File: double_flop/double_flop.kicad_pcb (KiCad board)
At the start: 2 copper layers, 55.8 x 70 mm, 8 parts, among them J1 Conn_01x04, SW1 Button 1, SW2 Button 2, SW3 Button 3, SW4 Button 4, U1 STM32F401, U2 CR2013-MI2120

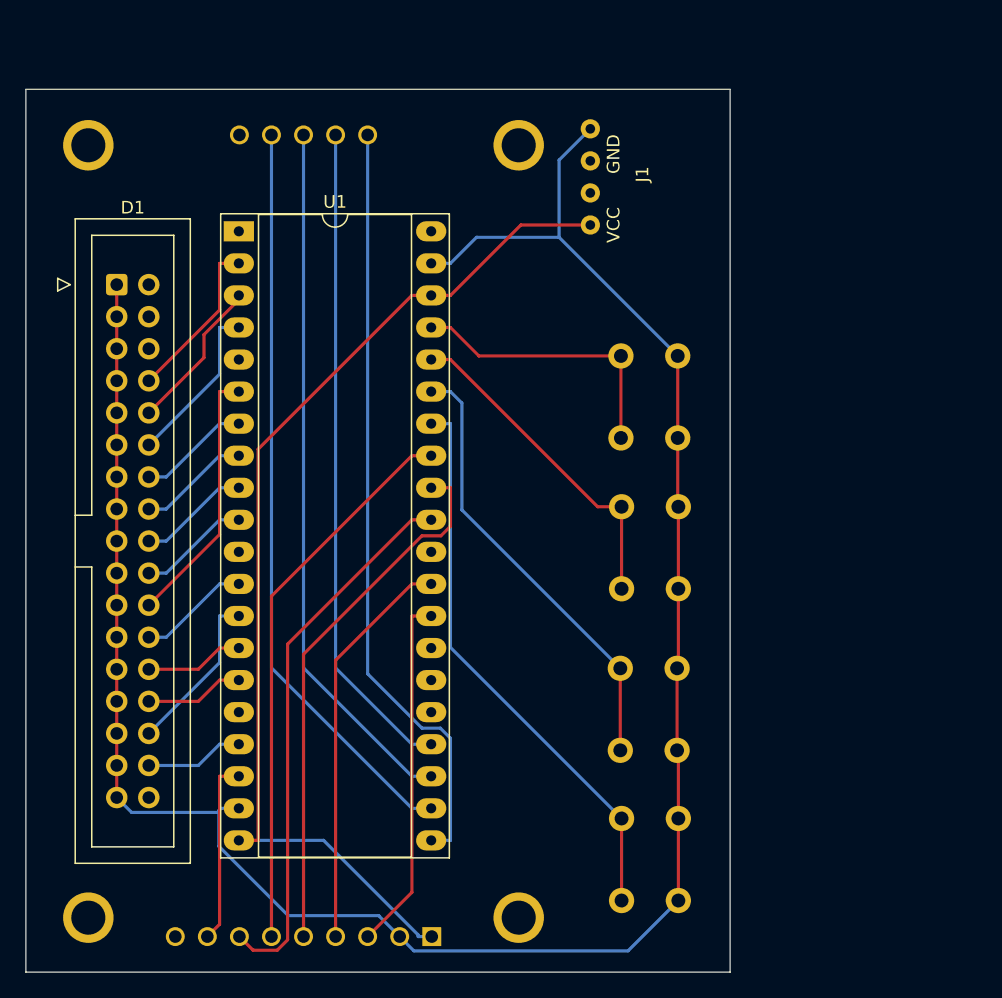
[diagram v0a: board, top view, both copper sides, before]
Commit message: Update 08042024
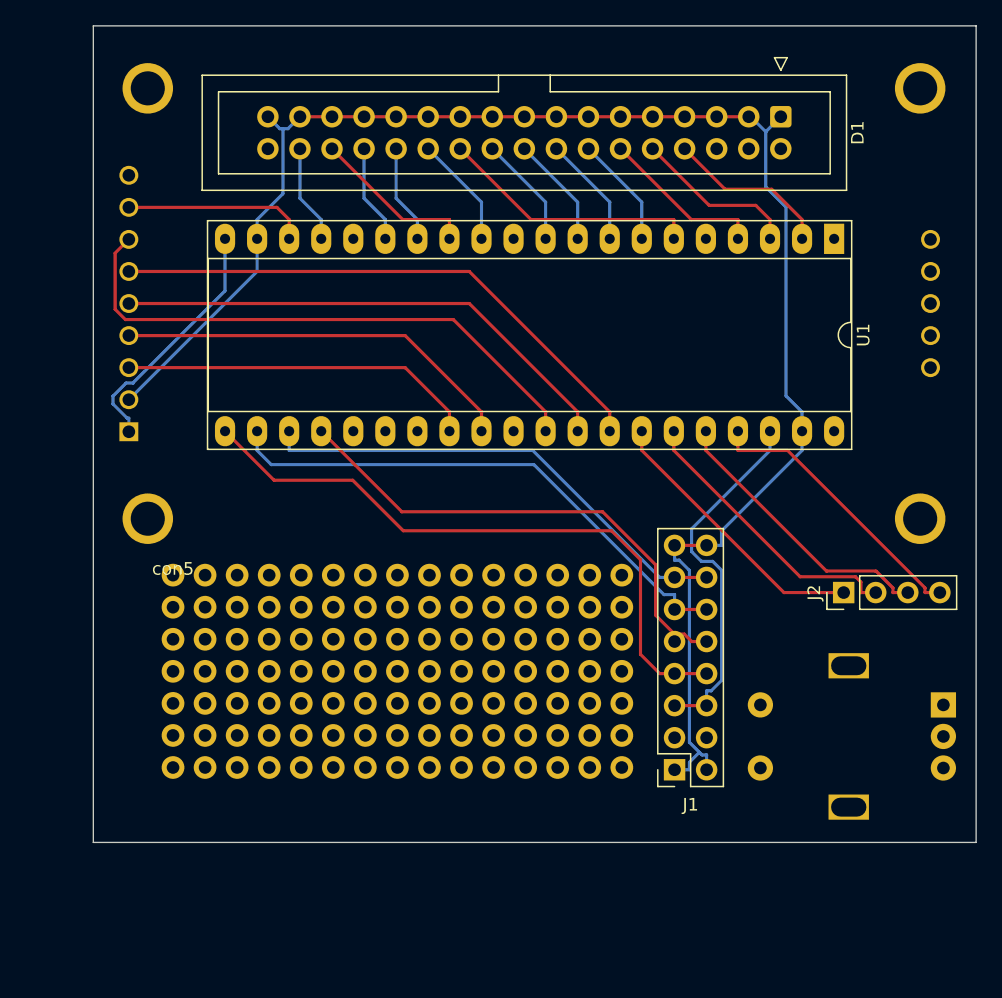
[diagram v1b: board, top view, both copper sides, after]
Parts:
- removed SW1: Button 1, Button_Switch_THT:SW_PUSH_6mm
- removed SW2: Button 2, Button_Switch_THT:SW_PUSH_6mm
- removed SW3: Button 3, Button_Switch_THT:SW_PUSH_6mm
- removed SW4: Button 4, Button_Switch_THT:SW_PUSH_6mm
- added J2: Conn_01x04_Pin, Double_flop_lib:PinHeader_1x04_P2.54mm_Vertical, F.Cu at (193.9, 67.5)
- added con5: Devboard, Double_flop:Devboard, F.Cu at (140.8, 66.1)
- added con6: RotaryEncoder_Alps_EC11E-Switch_Vertical_H20mm, Double_flop_lib:RotaryEncoder_Alps_EC11E-Switch_Vertical_H20mm, B.Cu at (201.8, 76.4)
- D1: footprint Connector_IDC:IDC-Header_2x17_P2.54mm_Vertical -> Double_flop_lib:IDC-Header_2x17_P2.54mm_Vertical
- J1: value Conn_01x04 -> SDCard Adapter; footprint Double_flop:USB-C Power board -> Double_flop_lib:PinSocket_2x08_P2.54mm_Vertical
- U1: footprint Package_DIP:DIP-40_W15.24mm_Socket_LongPads -> Double_flop_lib:DIP-40_W15.24mm_Socket_LongPads
- U2: footprint Display:CR2013-MI2120 -> Double_flop_lib:CR2013-MI2120
- moved D1 54.3 mm to (188.9, 29.8), turned to -90 degrees
- moved J1 47.5 mm to (180.5, 81.5), turned to 180 degrees
- moved U1 47.2 mm to (193.1, 39.5), turned to -90 degrees
- moved U2 46.6 mm to (137.3, 54.8), turned to 0 degrees
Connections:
- J1 pad 1: +5V -> GND
- J1 pad 2: unconnected-(J1-Pin_2-Pad2) -> GND
- J1 pad 4: GND -> unconnected-(J1-Pin_4-Pad4)
- U1 pad 20: +5V -> Net-(U2-VCC)
- U2 pad 1: +5V -> Net-(U2-VCC)
- U2 pad 10: SS -> unconnected-(U2-SD_CS-Pad10)
- U2 pad 11: MOSI -> unconnected-(U2-SD_MOSI-Pad11)
- U2 pad 12: MISO -> unconnected-(U2-SD_MISO-Pad12)
- U2 pad 13: SCK -> unconnected-(U2-SD_SCK-Pad13)
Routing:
- net +5V: track 84.7 -> 29.1 mm
- net GND: track 172.4 -> 131.4 mm
- net Net-(J2-Pin_1): track 44.9 -> 22.2 mm
- net Net-(U2-VCC): track 0.00 -> 19.9 mm
- net MISO: track 55.9 -> 38.8 mm
- net SCK: track 59.5 -> 43.1 mm
- net Net-(J2-Pin_2): track 35.5 -> 22.7 mm
- net MOSI: track 52.3 -> 40.4 mm
- net SS: track 61.0 -> 50.5 mm
- net Net-(J2-Pin_3): track 26.4 -> 22.4 mm
- net tft_dc: track 42.8 -> 40.6 mm
- net tft_sck: track 43.5 -> 45.0 mm
- net Net-(D1-MOTOR_0): track 12.3 -> 13.2 mm
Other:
- board size 55.8 x 70 mm -> 70 x 64.7 mm
